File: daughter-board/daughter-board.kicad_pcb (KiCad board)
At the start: 2 copper layers, 50 x 15 mm, 10 parts, among them J1 USB-C Connector, J2 Ribbon Connector, P1 IPOD_CONNECTOR_MALE, U1 AP2331SA-7

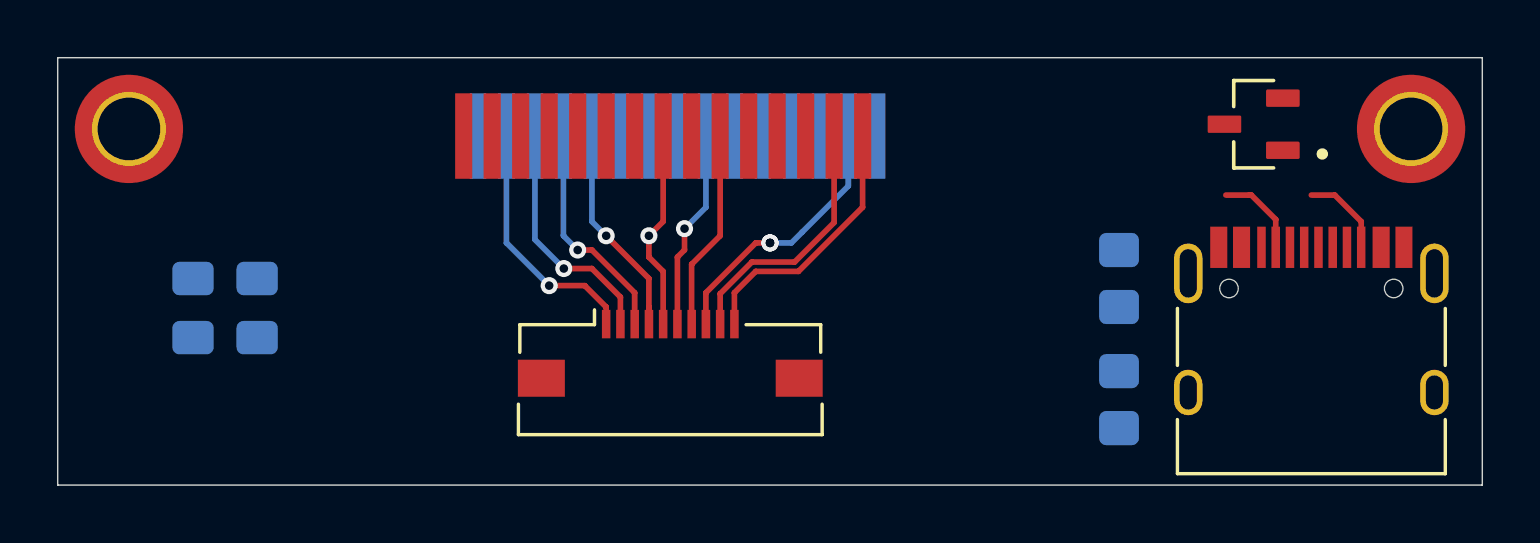
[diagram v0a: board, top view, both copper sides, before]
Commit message: Eh, not sure about this.
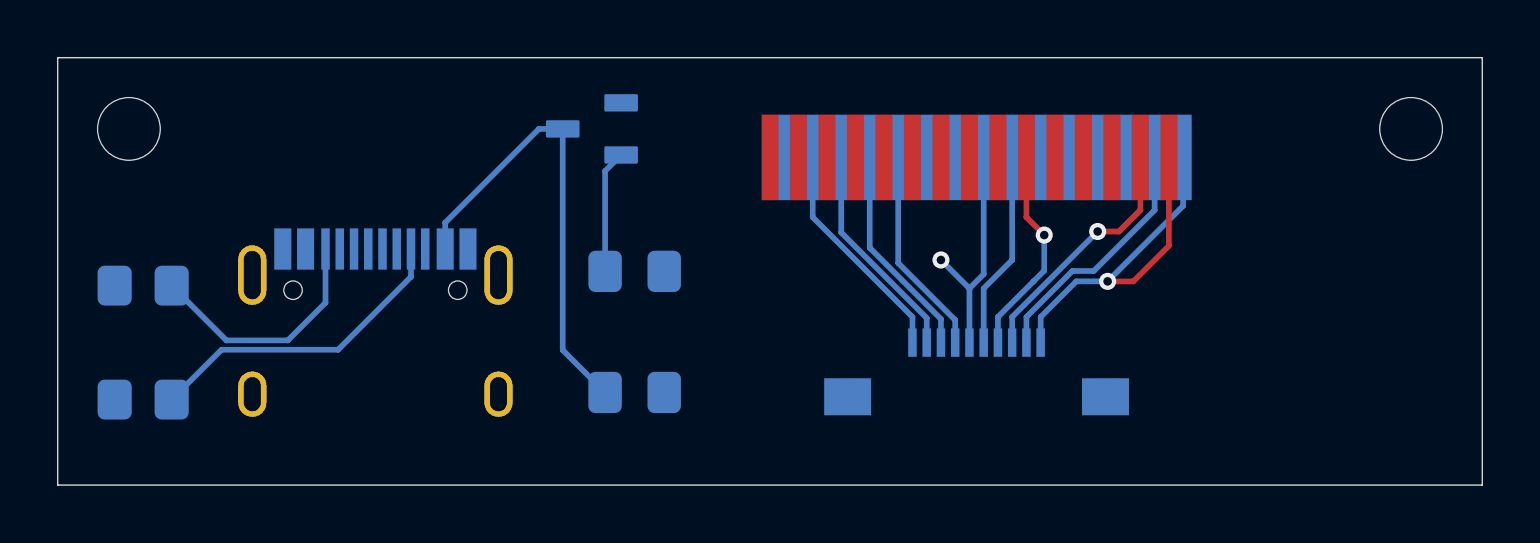
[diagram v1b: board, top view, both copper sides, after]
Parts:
- J1, J2, U1: moved to B.Cu
- REF** (x2): value MountingHole_2.2mm_M2_DIN965_Pad_TopOnly -> MountingHole_2.2mm_M2; footprint MountingHole:MountingHole_2.2mm_M2_DIN965_Pad_TopOnly -> MountingHole:MountingHole_2.2mm_M2
- moved R2 34.5 mm to (158.5, 99.8), turned to 180 degrees
- moved R1 34.5 mm to (158.5, 95.8), turned to 180 degrees
- moved J1 32.9 mm to (166.7, 98.5), turned to 180 degrees
- moved U1 23.2 mm to (174.2, 90.2)
- moved C1 15.8 mm to (175.8, 99.5), turned to 0 degrees
- moved C2 13.3 mm to (175.8, 95.2), turned to 0 degrees
- moved P1 10.8 mm to (187.5, 91.2)
- moved J2 10.8 mm to (187.8, 98.8), turned to 180 degrees
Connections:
- J2 pad 1: D+ -> GNDA
- J2 pad 10: GNDA -> D+
- J2 pad 2: D- -> OUT_R
- J2 pad 3: +5V -> OUT_L
- J2 pad 4: ACC -> TX
- J2 pad 5: GNDS -> RX
- J2 pad 6: RX -> GNDS
- J2 pad 7: TX -> ACC
- J2 pad 8: OUT_R -> +5V
- J2 pad 9: OUT_L -> D-
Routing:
- net Net-(U1-IN): track 0.00 -> 16.3 mm
- net Net-(J1-CC1): track 3.08 -> 11.2 mm
- net GNDA: track 9.34 -> 15.1 mm, vias 0 -> 1
- net Net-(J1-CC2): track 3.11 -> 8.63 mm
- net +5V: track 7.93 -> 12.0 mm, vias 1 -> 0
- net GNDS: track 7.01 -> 8.22 mm
- net D+: track 8.78 -> 8.05 mm, vias 1 -> 0
- net TX: track 7.01 -> 7.71 mm, vias 0 -> 1
- net ACC: track 8.03 -> 7.43 mm, vias 1 -> 0
- net D-: track 8.42 -> 7.84 mm, vias 1 -> 0
- net OUT_R: track 9.40 -> 8.90 mm, vias 2 -> 0
- net OUT_L: track 9.14 -> 8.90 mm, vias 0 -> 1
- net RX: vias 1 -> 0
